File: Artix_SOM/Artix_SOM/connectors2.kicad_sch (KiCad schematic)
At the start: 1 part

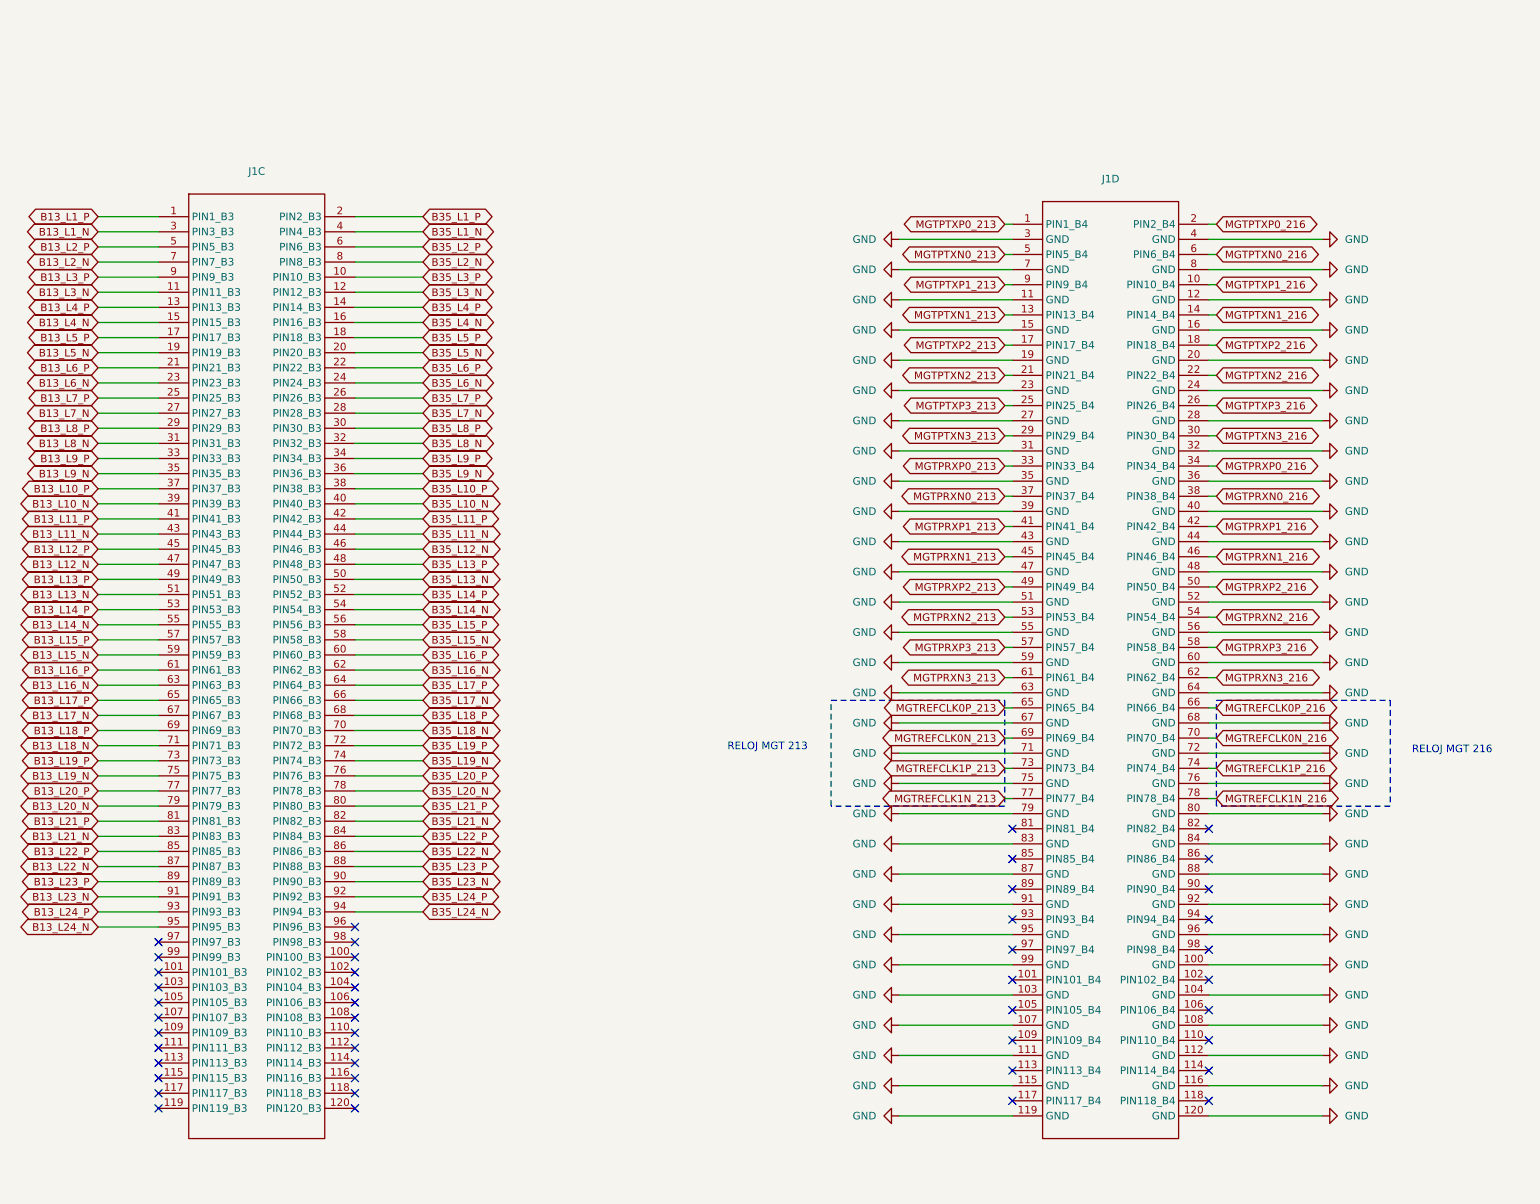
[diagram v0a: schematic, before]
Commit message: update
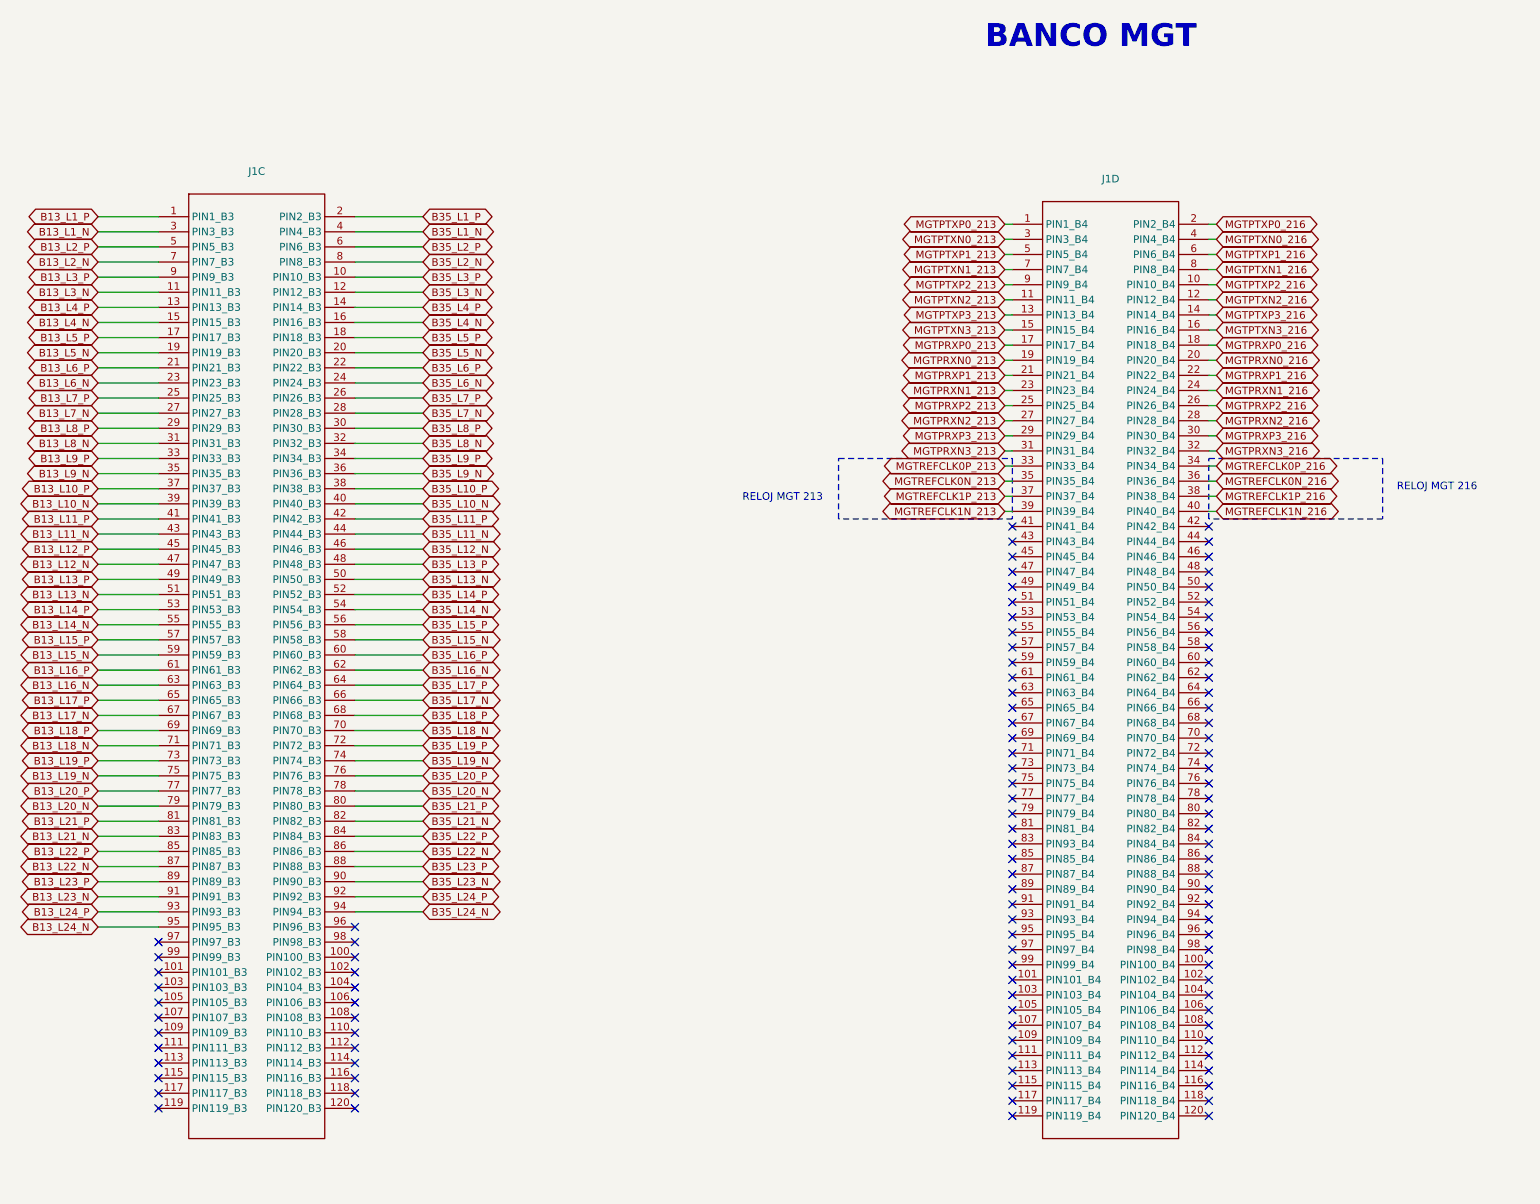
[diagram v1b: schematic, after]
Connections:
- net MGTPRXN0_213: now also J1.19 (PIN19_B4); no longer J1.37 (PIN37_B4)
- net MGTPRXN0_216: now also J1.20 (PIN20_B4); no longer J1.38 (PIN38_B4)
- net MGTPRXN1_213: now also J1.23 (PIN23_B4); no longer J1.45 (PIN45_B4)
- net MGTPRXN1_216: now also J1.24 (PIN24_B4); no longer J1.46 (PIN46_B4)
- net MGTPRXN2_213: now also J1.27 (PIN27_B4); no longer J1.53 (PIN53_B4)
- net MGTPRXN2_216: now also J1.28 (PIN28_B4); no longer J1.54 (PIN54_B4)
- net MGTPRXN3_213: now also J1.31 (PIN31_B4); no longer J1.61 (PIN61_B4)
- net MGTPRXN3_216: now also J1.32 (PIN32_B4); no longer J1.62 (PIN62_B4)
- net MGTPRXP0_213: now also J1.17 (PIN17_B4); no longer J1.33 (PIN33_B4)
- net MGTPRXP0_216: now also J1.18 (PIN18_B4); no longer J1.34 (PIN34_B4)
- net MGTPRXP1_213: now also J1.21 (PIN21_B4); no longer J1.41 (PIN41_B4)
- net MGTPRXP1_216: now also J1.22 (PIN22_B4); no longer J1.42 (PIN42_B4)
- net MGTPRXP2_213: now also J1.25 (PIN25_B4); no longer J1.49 (PIN49_B4)
- net MGTPRXP2_216: now also J1.26 (PIN26_B4); no longer J1.50 (PIN50_B4)
- net MGTPRXP3_213: now also J1.29 (PIN29_B4); no longer J1.57 (PIN57_B4)
- net MGTPRXP3_216: now also J1.30 (PIN30_B4); no longer J1.58 (PIN58_B4)
- net MGTPTXN0_213: now also J1.3 (PIN3_B4); no longer J1.5 (PIN5_B4)
- net MGTPTXN0_216: now also J1.4 (PIN4_B4); no longer J1.6 (PIN6_B4)
- net MGTPTXN1_213: now also J1.7 (PIN7_B4); no longer J1.13 (PIN13_B4)
- net MGTPTXN1_216: now also J1.8 (PIN8_B4); no longer J1.14 (PIN14_B4)
- net MGTPTXN2_213: now also J1.11 (PIN11_B4); no longer J1.21 (PIN21_B4)
- net MGTPTXN2_216: now also J1.12 (PIN12_B4); no longer J1.22 (PIN22_B4)
- net MGTPTXN3_213: now also J1.15 (PIN15_B4); no longer J1.29 (PIN29_B4)
- net MGTPTXN3_216: now also J1.16 (PIN16_B4); no longer J1.30 (PIN30_B4)
- net MGTPTXP1_213: now also J1.5 (PIN5_B4); no longer J1.9 (PIN9_B4)
- net MGTPTXP1_216: now also J1.6 (PIN6_B4); no longer J1.10 (PIN10_B4)
- net MGTPTXP2_213: now also J1.9 (PIN9_B4); no longer J1.17 (PIN17_B4)
- net MGTPTXP2_216: now also J1.10 (PIN10_B4); no longer J1.18 (PIN18_B4)
- net MGTPTXP3_213: now also J1.13 (PIN13_B4); no longer J1.25 (PIN25_B4)
- net MGTPTXP3_216: now also J1.14 (PIN14_B4); no longer J1.26 (PIN26_B4)
- net MGTREFCLK0N_213: now also J1.35 (PIN35_B4); no longer J1.69 (PIN69_B4)
- net MGTREFCLK0N_216: now also J1.36 (PIN36_B4); no longer J1.70 (PIN70_B4)
- net MGTREFCLK0P_213: now also J1.33 (PIN33_B4); no longer J1.65 (PIN65_B4)
- net MGTREFCLK0P_216: now also J1.34 (PIN34_B4); no longer J1.66 (PIN66_B4)
- net MGTREFCLK1N_213: now also J1.39 (PIN39_B4); no longer J1.77 (PIN77_B4)
- net MGTREFCLK1N_216: now also J1.40 (PIN40_B4); no longer J1.78 (PIN78_B4)
- net MGTREFCLK1P_213: now also J1.37 (PIN37_B4); no longer J1.73 (PIN73_B4)
- net MGTREFCLK1P_216: now also J1.38 (PIN38_B4); no longer J1.74 (PIN74_B4)
- removed net GND: J1.100 (GND), J1.103 (GND), J1.104 (GND), J1.107 (GND), J1.108 (GND), J1.11 (GND), J1.111 (GND), J1.112 (GND), J1.115 (GND), J1.116 (GND), J1.119 (GND), J1.12 (GND), J1.120 (GND), J1.15 (GND), J1.16 (GND), J1.19 (GND), J1.20 (GND), J1.23 (GND), J1.24 (GND), J1.27 (GND), J1.28 (GND), J1.3 (GND), J1.31 (GND), J1.32 (GND), J1.35 (GND), J1.36 (GND), J1.39 (GND), J1.4 (GND), J1.40 (GND), J1.43 (GND), J1.44 (GND), J1.47 (GND), J1.48 (GND), J1.51 (GND), J1.52 (GND), J1.55 (GND), J1.56 (GND), J1.59 (GND), J1.60 (GND), J1.63 (GND), J1.64 (GND), J1.67 (GND), J1.68 (GND), J1.7 (GND), J1.71 (GND), J1.72 (GND), J1.75 (GND), J1.76 (GND), J1.79 (GND), J1.8 (GND), J1.80 (GND), J1.83 (GND), J1.84 (GND), J1.87 (GND), J1.88 (GND), J1.91 (GND), J1.92 (GND), J1.95 (GND), J1.96 (GND), J1.99 (GND)
- no-connect marks 45 -> 105
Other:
- note added: "BANCO MGT"

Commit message: update
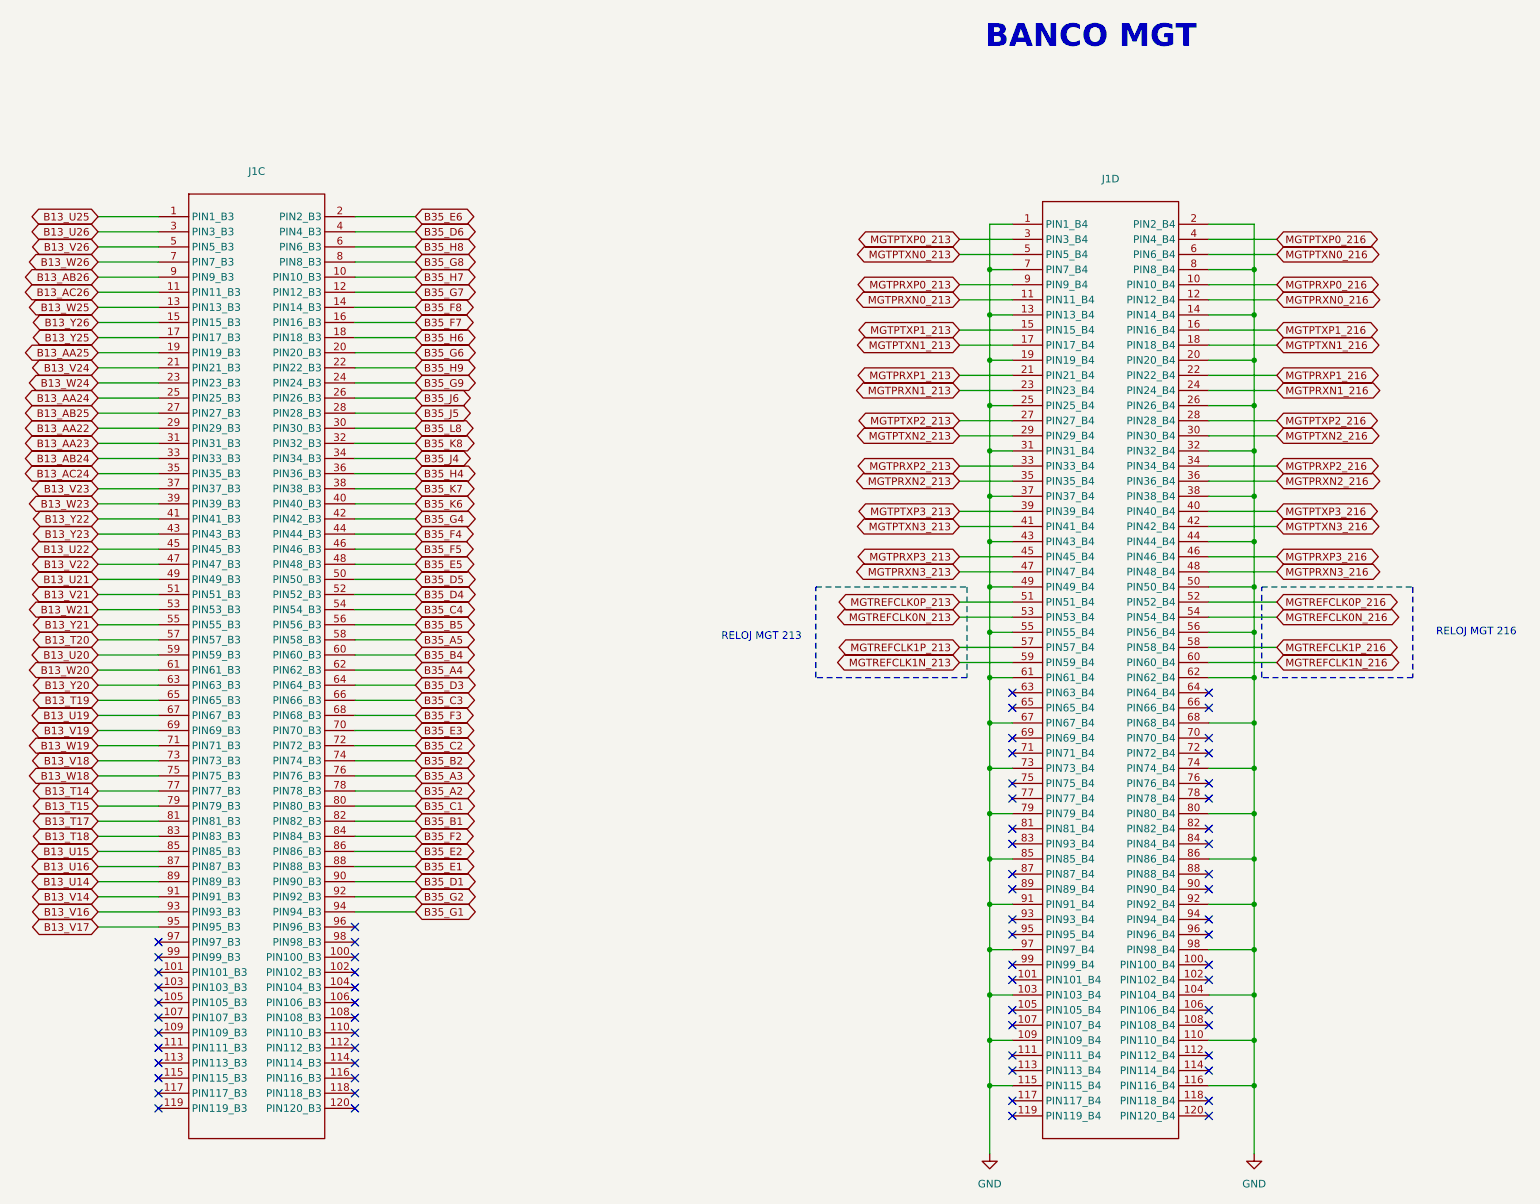
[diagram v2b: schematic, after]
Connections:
- net MGTPRXN0_213: now also J1.11 (PIN11_B4); no longer J1.19 (PIN19_B4)
- net MGTPRXN0_216: now also J1.12 (PIN12_B4); no longer J1.20 (PIN20_B4)
- net MGTPRXN2_213: now also J1.35 (PIN35_B4); no longer J1.27 (PIN27_B4)
- net MGTPRXN2_216: now also J1.36 (PIN36_B4); no longer J1.28 (PIN28_B4)
- net MGTPRXN3_213: now also J1.47 (PIN47_B4); no longer J1.31 (PIN31_B4)
- net MGTPRXN3_216: now also J1.48 (PIN48_B4); no longer J1.32 (PIN32_B4)
- net MGTPRXP0_213: now also J1.9 (PIN9_B4); no longer J1.17 (PIN17_B4)
- net MGTPRXP0_216: now also J1.10 (PIN10_B4); no longer J1.18 (PIN18_B4)
- net MGTPRXP2_213: now also J1.33 (PIN33_B4); no longer J1.25 (PIN25_B4)
- net MGTPRXP2_216: now also J1.34 (PIN34_B4); no longer J1.26 (PIN26_B4)
- net MGTPRXP3_213: now also J1.45 (PIN45_B4); no longer J1.29 (PIN29_B4)
- net MGTPRXP3_216: now also J1.46 (PIN46_B4); no longer J1.30 (PIN30_B4)
- net MGTPTXN0_213: now also J1.5 (PIN5_B4); no longer J1.3 (PIN3_B4)
- net MGTPTXN0_216: now also J1.6 (PIN6_B4); no longer J1.4 (PIN4_B4)
- net MGTPTXN1_213: now also J1.17 (PIN17_B4); no longer J1.7 (PIN7_B4)
- net MGTPTXN1_216: now also J1.18 (PIN18_B4); no longer J1.8 (PIN8_B4)
- net MGTPTXN2_213: now also J1.29 (PIN29_B4); no longer J1.11 (PIN11_B4)
- net MGTPTXN2_216: now also J1.30 (PIN30_B4); no longer J1.12 (PIN12_B4)
- net MGTPTXN3_213: now also J1.41 (PIN41_B4); no longer J1.15 (PIN15_B4)
- net MGTPTXN3_216: now also J1.42 (PIN42_B4); no longer J1.16 (PIN16_B4)
- net MGTPTXP0_213: now also J1.3 (PIN3_B4); no longer J1.1 (PIN1_B4)
- net MGTPTXP0_216: now also J1.4 (PIN4_B4); no longer J1.2 (PIN2_B4)
- net MGTPTXP1_213: now also J1.15 (PIN15_B4); no longer J1.5 (PIN5_B4)
- net MGTPTXP1_216: now also J1.16 (PIN16_B4); no longer J1.6 (PIN6_B4)
- net MGTPTXP2_213: now also J1.27 (PIN27_B4); no longer J1.9 (PIN9_B4)
- net MGTPTXP2_216: now also J1.28 (PIN28_B4); no longer J1.10 (PIN10_B4)
- net MGTPTXP3_213: now also J1.39 (PIN39_B4); no longer J1.13 (PIN13_B4)
- net MGTPTXP3_216: now also J1.40 (PIN40_B4); no longer J1.14 (PIN14_B4)
- net MGTREFCLK0N_213: now also J1.53 (PIN53_B4); no longer J1.35 (PIN35_B4)
- net MGTREFCLK0N_216: now also J1.54 (PIN54_B4); no longer J1.36 (PIN36_B4)
- net MGTREFCLK0P_213: now also J1.51 (PIN51_B4); no longer J1.33 (PIN33_B4)
- net MGTREFCLK0P_216: now also J1.52 (PIN52_B4); no longer J1.34 (PIN34_B4)
- net MGTREFCLK1N_213: now also J1.59 (PIN59_B4); no longer J1.39 (PIN39_B4)
- net MGTREFCLK1N_216: now also J1.60 (PIN60_B4); no longer J1.40 (PIN40_B4)
- net MGTREFCLK1P_213: now also J1.57 (PIN57_B4); no longer J1.37 (PIN37_B4)
- net MGTREFCLK1P_216: now also J1.58 (PIN58_B4); no longer J1.38 (PIN38_B4)
- net GND: now reaches J1.103 (PIN103_B4)
- net GND: now also J1.1 (PIN1_B4), J1.104 (PIN104_B4), J1.109 (PIN109_B4), J1.110 (PIN110_B4), J1.115 (PIN115_B4), J1.116 (PIN116_B4), J1.13 (PIN13_B4), J1.14 (PIN14_B4), J1.19 (PIN19_B4), J1.2 (PIN2_B4), J1.20 (PIN20_B4), J1.25 (PIN25_B4), J1.26 (PIN26_B4), J1.31 (PIN31_B4), J1.32 (PIN32_B4), J1.37 (PIN37_B4), J1.38 (PIN38_B4), J1.43 (PIN43_B4), J1.44 (PIN44_B4), J1.49 (PIN49_B4), J1.50 (PIN50_B4), J1.55 (PIN55_B4), J1.56 (PIN56_B4), J1.61 (PIN61_B4), J1.62 (PIN62_B4), J1.67 (PIN67_B4), J1.68 (PIN68_B4), J1.7 (PIN7_B4), J1.73 (PIN73_B4), J1.74 (PIN74_B4), J1.79 (PIN79_B4), J1.8 (PIN8_B4), J1.80 (PIN80_B4), J1.85 (PIN85_B4), J1.86 (PIN86_B4), J1.91 (PIN91_B4), J1.92 (PIN92_B4), J1.97 (PIN97_B4), J1.98 (PIN98_B4)
- net B13_L10_N renamed B13_W23
- net B13_L10_P renamed B13_V23
- net B13_L11_N renamed B13_Y23
- net B13_L11_P renamed B13_Y22
- net B13_L12_N renamed B13_V22
- net B13_L12_P renamed B13_U22
- net B13_L13_N renamed B13_V21
- net B13_L13_P renamed B13_U21
- net B13_L14_N renamed B13_Y21
- net B13_L14_P renamed B13_W21
- net B13_L15_N renamed B13_U20
- net B13_L15_P renamed B13_T20
- net B13_L16_N renamed B13_Y20
- net B13_L16_P renamed B13_W20
- net B13_L17_N renamed B13_U19
- net B13_L17_P renamed B13_T19
- net B13_L18_N renamed B13_W19
- net B13_L18_P renamed B13_V19
- net B13_L19_N renamed B13_W18
- net B13_L19_P renamed B13_V18
- net B13_L1_N renamed B13_U26
- net B13_L1_P renamed B13_U25
- net B13_L20_N renamed B13_T15
- net B13_L20_P renamed B13_T14
- net B13_L21_N renamed B13_T18
- net B13_L21_P renamed B13_T17
- net B13_L22_N renamed B13_U16
- net B13_L22_P renamed B13_U15
- net B13_L23_N renamed B13_V14
- net B13_L23_P renamed B13_U14
- net B13_L24_N renamed B13_V17
- net B13_L24_P renamed B13_V16
- net B13_L2_N renamed B13_W26
- net B13_L2_P renamed B13_V26
- net B13_L3_N renamed B13_AC26
- net B13_L3_P renamed B13_AB26
- net B13_L4_N renamed B13_Y26
- net B13_L4_P renamed B13_W25
- net B13_L5_N renamed B13_AA25
- net B13_L5_P renamed B13_Y25
- net B13_L6_N renamed B13_W24
- net B13_L6_P renamed B13_V24
- net B13_L7_N renamed B13_AB25
- net B13_L7_P renamed B13_AA24
- net B13_L8_N renamed B13_AA23
- net B13_L8_P renamed B13_AA22
- net B13_L9_N renamed B13_AC24
- net B13_L9_P renamed B13_AB24
- net B35_L10_N renamed B35_K6
- net B35_L10_P renamed B35_K7
- net B35_L11_N renamed B35_F4
- net B35_L11_P renamed B35_G4
- net B35_L12_N renamed B35_F5
- net B35_L13_N renamed B35_D5
- net B35_L13_P renamed B35_E5
- net B35_L14_N renamed B35_C4
- net B35_L14_P renamed B35_D4
- net B35_L15_N renamed B35_A5
- net B35_L15_P renamed B35_B5
- net B35_L16_N renamed B35_A4
- net B35_L16_P renamed B35_B4
- net B35_L17_N renamed B35_C3
- net B35_L17_P renamed B35_D3
- net B35_L18_N renamed B35_E3
- net B35_L18_P renamed B35_F3
- net B35_L19_N renamed B35_B2
- net B35_L19_P renamed B35_C2
- net B35_L1_N renamed B35_D6
- net B35_L1_P renamed B35_E6
- net B35_L20_N renamed B35_A2
- net B35_L20_P renamed B35_A3
- net B35_L21_N renamed B35_B1
- net B35_L21_P renamed B35_C1
- net B35_L22_N renamed B35_E2
- net B35_L22_P renamed B35_F2
- net B35_L23_N renamed B35_D1
- net B35_L23_P renamed B35_E1
- net B35_L24_N renamed B35_G1
- net B35_L24_P renamed B35_G2
- net B35_L2_N renamed B35_G8
- net B35_L2_P renamed B35_H8
- net B35_L3_N renamed B35_G7
- net B35_L3_P renamed B35_H7
- net B35_L4_N renamed B35_F7
- net B35_L4_P renamed B35_F8
- net B35_L5_N renamed B35_G6
- net B35_L5_P renamed B35_H6
- net B35_L6_N renamed B35_G9
- net B35_L6_P renamed B35_H9
- net B35_L7_N renamed B35_J5
- net B35_L7_P renamed B35_J6
- net B35_L8_N renamed B35_K8
- net B35_L8_P renamed B35_L8
- net B35_L9_N renamed B35_H4
- net B35_L9_P renamed B35_J4
- no-connect marks 105 -> 65
